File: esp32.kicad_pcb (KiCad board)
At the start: 2 copper layers, 44 x 80 mm, 102 parts, among them J1 USB_C, J14 PWR_CONN, J15 SPI_0, J16 SPI_1, J3 A0, J4 A1, J5 A2, J6 D0, J7 D1, J8 USB_VOUT, Q10 AO3400A, Q11 AO3400A, Q12 AO3400A, Q3 AO3400A, Q4 AO3400A, Q5 AO3400A, Q6 AO3400A, Q7 AO3400A, Q8 AO3400A, Q9 AO3400A, SW1 SW_RST, SW2 SW_BOOT, U1 LMR36520ADDAR, U3 ESP32-S3-WROOM-1

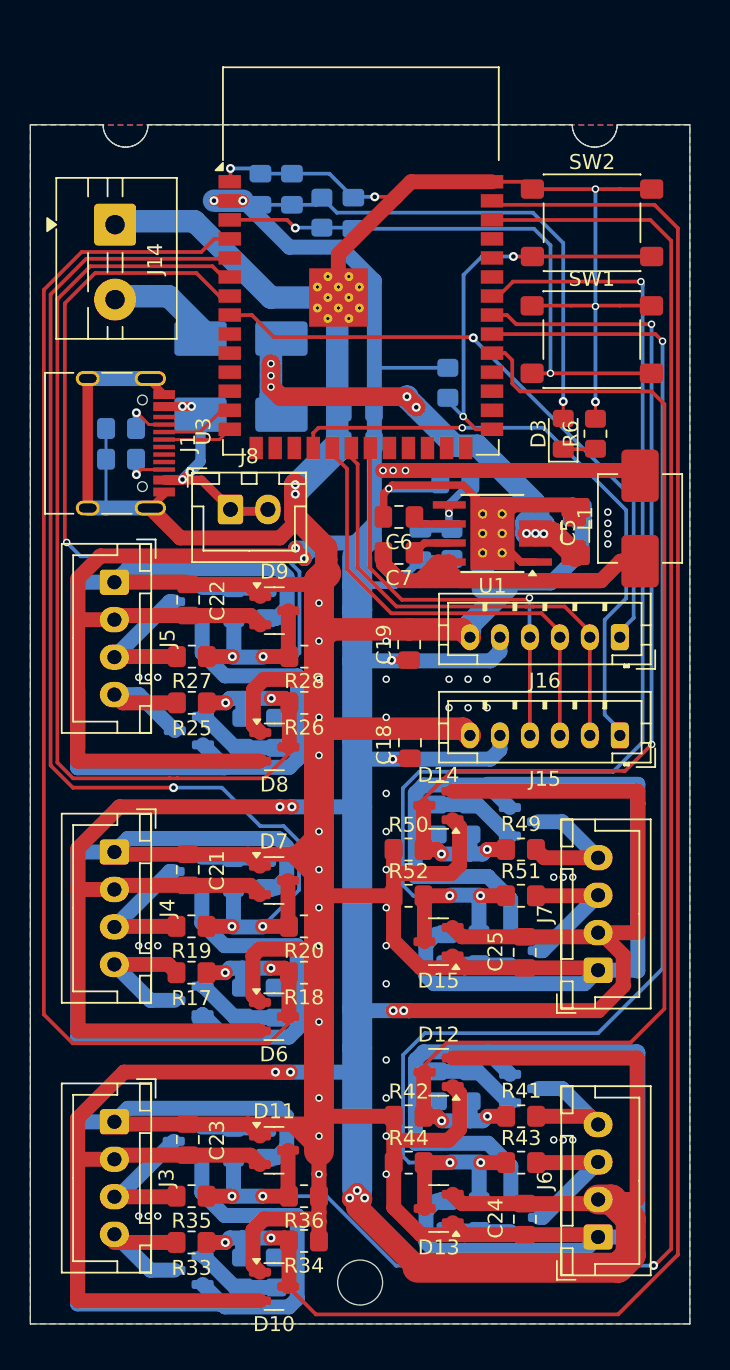
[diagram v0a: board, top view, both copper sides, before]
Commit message: review passed
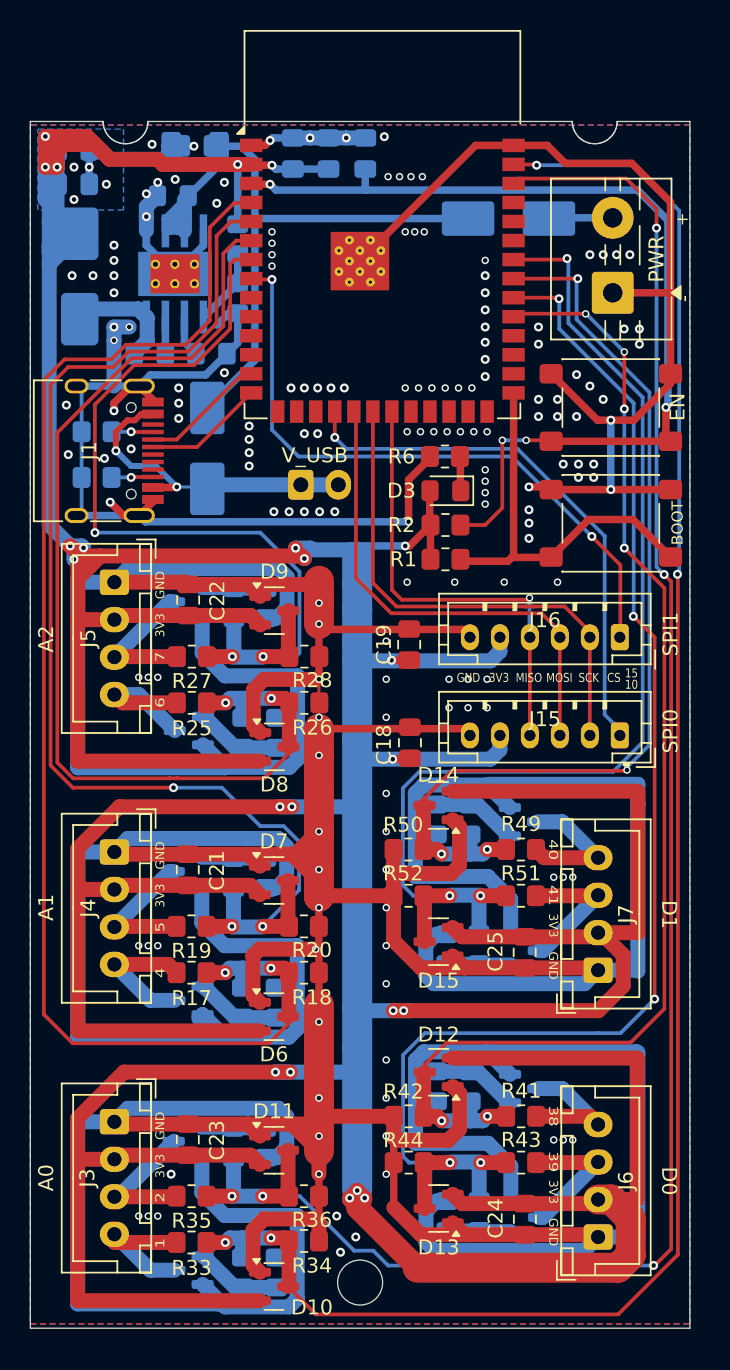
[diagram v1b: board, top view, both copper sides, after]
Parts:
- removed C12: 20pF, Capacitor_SMD:C_0805_2012Metric_Pad1.18x1.45mm_HandSolder
- removed J14: PWR_CONN, TerminalBlock:TerminalBlock_MaiXu_MX126-5.0-02P_1x02_P5.00mm
- removed SW1: SW_RST, Button_Switch_SMD:SW_SPST_PTS645Sx43SMTR92
- removed SW2: SW_BOOT, Button_Switch_SMD:SW_SPST_PTS645Sx43SMTR92
- added BOOT: SW_BOOT, Button_Switch_SMD:SW_SPST_PTS645Sx43SMTR92, F.Cu at (109.6, 97.5)
- added EN: SW_RST, Button_Switch_SMD:SW_SPST_PTS645Sx43SMTR92, F.Cu at (109.6, 89.8)
- added PWR: PWR_CONN, TerminalBlock:TerminalBlock_MaiXu_MX126-5.0-02P_1x02_P5.00mm, F.Cu at (109.7, 82.2)
- C18, C19, C21, C22, C23, C24, C25: value 100n -> 100nF
- C4: value 4.7uF -> 2.2uF
- C5: footprint Library:C_1206&0805 -> LED_SMD:LED_0805_2012Metric_Pad1.15x1.40mm_HandSolder; moved to B.Cu
- C6, L1, U1: moved to B.Cu
- C7: value 0.1uF -> 100nF; moved to B.Cu
- R1, R2: moved to F.Cu
- moved L1 40.7 mm to (74.2, 81.1)
- moved C5 35.0 mm to (80.4, 75.7), turned to 180 degrees
- moved C4 34.4 mm to (81.9, 72.4), turned to 180 degrees
- moved U1 27.4 mm to (80.5, 80.9), turned to -90 degrees
- moved C8 27.2 mm to (73.8, 72.6), turned to 0 degrees
- moved R7 24.8 mm to (84.7, 78.6), turned to 90 degrees
- moved C11 24.3 mm to (73.8, 74.9), turned to 0 degrees
- moved R2 22.4 mm to (98.6, 97.7), turned to 0 degrees
- moved C7 21.3 mm to (78.8, 86.2)
- moved D1 19.6 mm to (102.8, 77.2), turned to 0 degrees
- moved R53 19.0 mm to (84.7, 82.5), turned to 90 degrees
- moved C6 16.6 mm to (83.0, 86.2), turned to 0 degrees
- moved R1 11.8 mm to (98.6, 99.9), turned to 0 degrees
- moved R6 10.2 mm to (98.5, 93.1), turned to 180 degrees
- moved D3 8.73 mm to (98.6, 95.4), turned to 180 degrees
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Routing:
- net GND: track 728.0 -> 690.4 mm, vias 59 -> 171
- net /EN: track 38.6 -> 64.4 mm, vias 2 -> 4
- net Net-(U1-SW): track 34.9 -> 11.9 mm
- net VCC: track 38.3 -> 48.5 mm, vias 8 -> 0
- net /A5: track 64.3 -> 59.5 mm
- net +3V3: track 468.3 -> 463.9 mm, vias 19 -> 22
- net /SPI_CS0: track 40.0 -> 35.8 mm
- net /D-: track 4.45 -> 8.38 mm
- net /D3: track 79.6 -> 76.4 mm
- net V_USB: track 19.6 -> 22.5 mm, vias 4 -> 2
- net /A2: track 90.3 -> 92.9 mm
- net /D+: track 5.62 -> 8.06 mm
- net Net-(D1-A): track 7.82 -> 5.40 mm
- net /A3: track 81.0 -> 83.4 mm
- net /D1: track 94.5 -> 92.2 mm, vias 3 -> 5
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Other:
- board size 44 x 80 mm -> 44 x 80.5 mm
- board text added: "+"
- board text added: "-"
- board text added: "1"
- board text added: "10"
- board text added: "15"
- board text added: "2"
- board text added: "38"
- board text added: "39"
- board text added: "3V3"
- board text added: "4"
- board text added: "40"
- board text added: "41"
- board text added: "5"
- board text added: "6"
- board text added: "7"
- board text added: "A0"
- board text added: "A1"
- board text added: "A2"
- board text added: "CS"
- board text added: "D0"
- board text added: "D1"
- board text added: "GND"
- board text added: "MISO"
- board text added: "MOSI"
- board text added: "SCK"
- board text added: "SPI0"
- board text added: "SPI1"
- board text added: "V_USB"
